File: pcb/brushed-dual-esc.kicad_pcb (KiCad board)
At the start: 2 copper layers, 30 x 25 mm, 33 parts, among them J2 TC2030-NL, J3 DRV1_OUT1, J4 Conn_01x04_Pin, J5 DRV1_OUT2, J6 DRV2_OUT1, J7 DRV2_OUT2, J8 +BATT, J9 -BATT, U1 AZ1117CH-5.0TRG1, U2 TLV77133PDBVR, U3 STM32C011F6U6, U6 DRV8231ADDAR, U7 DRV8231ADDAR

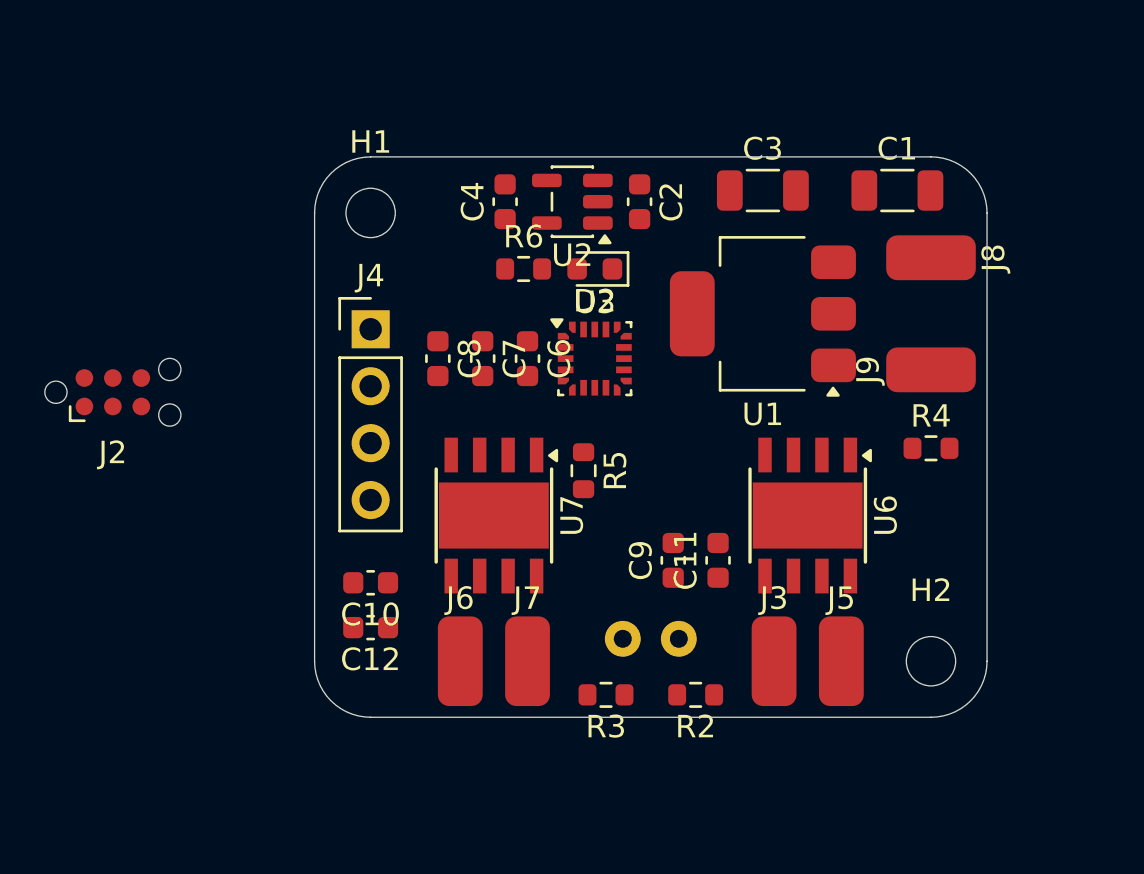
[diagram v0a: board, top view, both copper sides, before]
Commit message: New layout
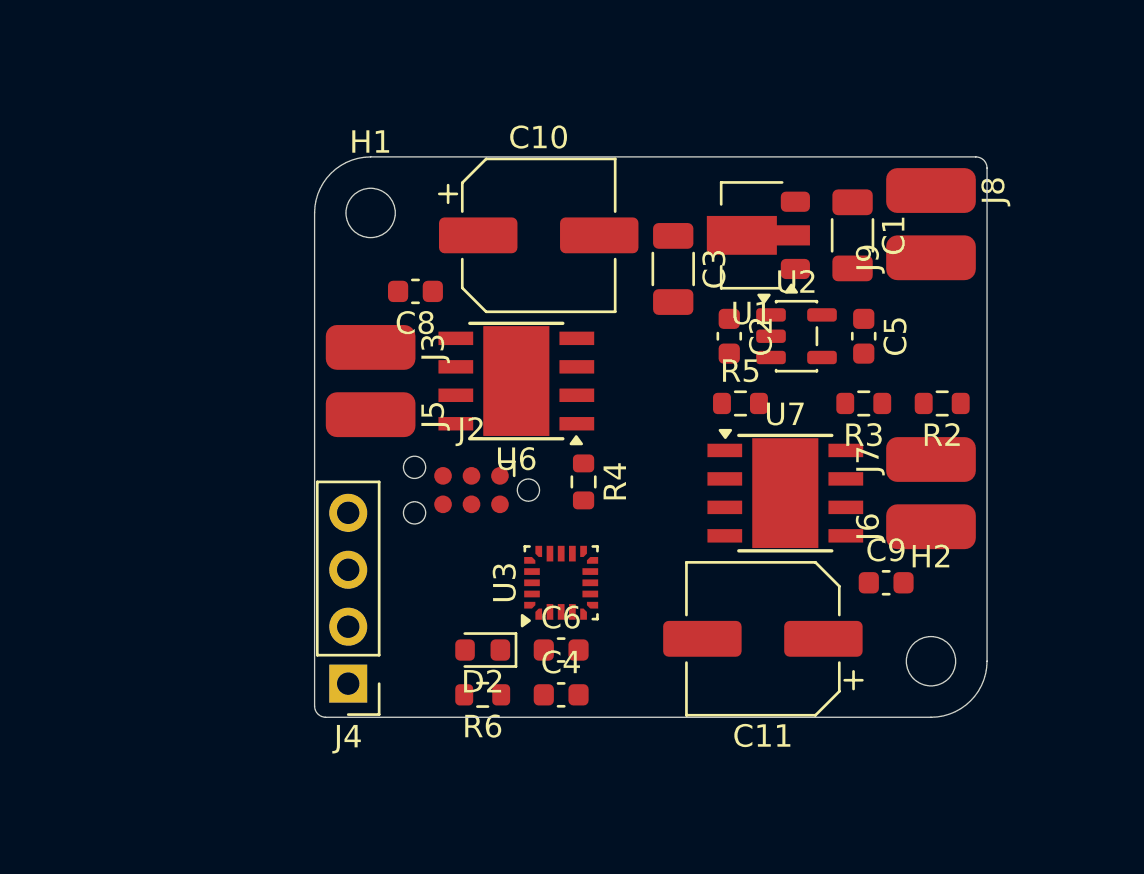
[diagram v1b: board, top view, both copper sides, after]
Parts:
- removed C12, C7: UMK107BJ105KA-T, Capacitor_SMD:C_0603_1608Metric
- C1, C3: value CL21A226KOQNNNG -> CL31A226KAHNNNE
- C10, C11: value UMK107BJ105KA-T -> A768EB107M1ELAS036; footprint Capacitor_SMD:C_0603_1608Metric -> Capacitor_SMD:CP_Elec_6.3x5.7
- C2, C4: value UMK107BJ105KA-T -> 4.7u
- C5: value A750EM337M1CAAE015 -> 4.7u; footprint Capacitor_THT:C_Radial_D6.3mm_H11.0mm_P2.50mm -> Capacitor_SMD:C_0603_1608Metric; moved to F.Cu
- C6, C8, C9: value UMK107BJ105KA-T -> 100n
- U1: value AZ1117CH-5.0TRG1 -> AZ1117CR-5.0TRG1; footprint Package_TO_SOT_SMD:SOT-223-3_TabPin2 -> Package_TO_SOT_SMD:SOT-89-3
- moved J5 23.7 mm to (147.5, 61.5), turned to -90 degrees
- moved J3 22.8 mm to (147.5, 58.5), turned to -90 degrees
- moved C4 22.1 mm to (156.0, 74.0), turned to 0 degrees
- moved J6 21.8 mm to (172.5, 66.5), turned to 90 degrees
- moved J7 20.1 mm to (172.5, 63.5), turned to 90 degrees
- moved R6 19.1 mm to (152.5, 74.0), turned to 180 degrees
- moved D2 17.7 mm to (152.5, 72.0)
- moved R3 17.4 mm to (169.5, 61.0)
- moved C10 17.2 mm to (155.0, 53.5), turned to 0 degrees
- moved R2 17.0 mm to (173.0, 61.0)
- moved J2 16.6 mm to (152.0, 64.9), turned to 180 degrees
- moved J4 15.8 mm to (146.5, 73.5), turned to 180 degrees
- moved C5 15.8 mm to (169.5, 58.0), turned to -90 degrees
- moved R4 15.6 mm to (157.0, 64.5), turned to -90 degrees
- moved U6 14.3 mm to (154.0, 60.0), turned to 180 degrees
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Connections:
- C5 pad 1: +BATT -> +3V3
- C8 pad 1: +3V3 -> +BATT
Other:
- outline, holes or cut-outs redrawn

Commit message: Begin routing
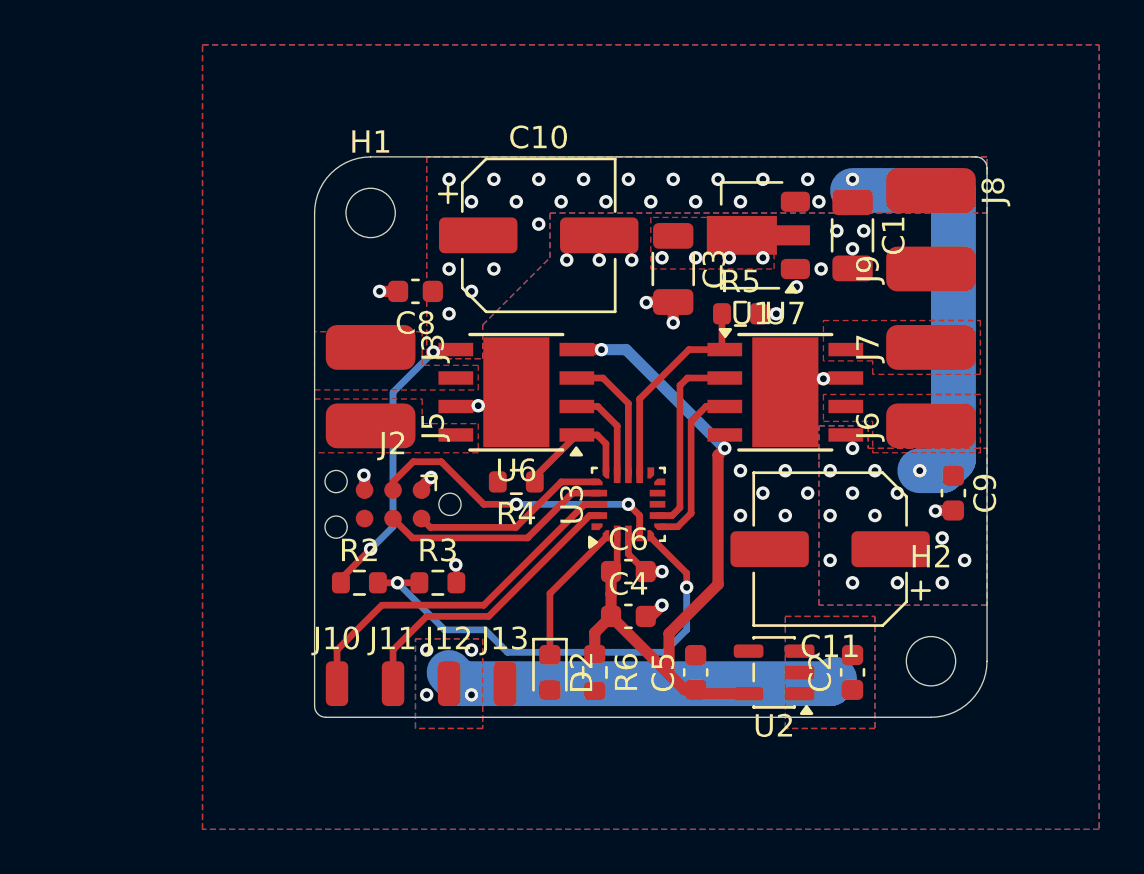
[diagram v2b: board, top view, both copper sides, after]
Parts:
- removed J4: Conn_01x04_Pin, Connector_PinHeader_2.54mm:PinHeader_1x04_P2.54mm_Vertical
- added J10: RX_CH2, Connector_Wire:SolderWirePad_1x01_SMD_1x2mm, F.Cu at (146.0, 73.5)
- added J11: RX_CH1, Connector_Wire:SolderWirePad_1x01_SMD_1x2mm, F.Cu at (148.5, 73.5)
- added J12: +5V, Connector_Wire:SolderWirePad_1x01_SMD_1x2mm, F.Cu at (151.0, 73.5)
- added J13: GND, Connector_Wire:SolderWirePad_1x01_SMD_1x2mm, F.Cu at (153.5, 73.5)
- moved R2 27.2 mm to (147.0, 69.0), turned to 0 degrees
- moved R3 20.6 mm to (150.5, 69.0), turned to 0 degrees
- moved C5 16.8 mm to (162.0, 73.0), turned to 90 degrees
- moved C2 16.0 mm to (169.0, 73.0), turned to 90 degrees
- moved U2 15.0 mm to (165.5, 73.0), turned to 180 degrees
- moved R6 5.10 mm to (157.5, 73.0), turned to -90 degrees
- moved C11 5.00 mm to (168.0, 67.5)
- moved C9 5.00 mm to (173.5, 65.0), turned to -90 degrees
- moved J7 5.00 mm to (172.5, 58.5)
- moved C4 4.61 mm to (159.0, 70.5)
- moved C6 4.61 mm to (159.0, 68.5)
- moved U3 4.61 mm to (159.0, 65.5)
- moved J6 4.50 mm to (172.5, 62.0)
- moved U7 4.50 mm to (166.0, 60.5)
- moved R5 4.00 mm to (164.0, 57.0)
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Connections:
- U3 pad 13: /DRV2_IN2 -> /DRV1_IN1
- U3 pad 14: /DRV2_IN1 -> /DRV1_IN2
- U3 pad 15: /BATT_SENSE -> /DRV1_ISENSE
- U3 pad 5: /DRV1_ISENSE -> /BATT_SENSE
- U3 pad 6: /DRV1_IN1 -> /DRV2_IN1
- U3 pad 7: /DRV1_IN2 -> /DRV2_IN2
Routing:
- net +3V3: track 0.00 -> 33.6 mm, vias 0 -> 3
- net +BATT: track 0.00 -> 31.3 mm, vias 0 -> 39
- net /BATT_SENSE: track 0.00 -> 21.2 mm, vias 0 -> 2
- net +5V: track 0.00 -> 17.5 mm, vias 0 -> 8
- net /RX_CH2: track 0.00 -> 15.9 mm
- net GND: track 0.00 -> 15.6 mm, vias 0 -> 25
- net /~{RESET}: track 0.00 -> 13.5 mm, vias 0 -> 2
- net /RX_CH1: track 0.00 -> 13.2 mm
- net /SWCLK: track 0.00 -> 10.4 mm
- net /DRV2_ISENSE: track 0.00 -> 9.76 mm
- net /SWDIO: track 0.00 -> 8.77 mm
- net /DRV2_IN2: track 0.00 -> 8.73 mm
- net /DRV2_IN1: track 0.00 -> 7.45 mm
- net /LED: track 0.00 -> 6.27 mm
- net /DRV1_IN1: track 0.00 -> 5.97 mm
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- added copper zone on B.Cu, net +5V
- added copper zone on F.Cu, net +5V
- added copper zone on B.Cu, net +BATT
- added copper zone on F.Cu, net +BATT
- added copper zone on F.Cu, net /DRV1_OUT1
- added copper zone on F.Cu, net /DRV1_OUT2
- added copper zone on F.Cu, net /DRV2_OUT1
- added copper zone on F.Cu, net /DRV2_OUT2
- added copper zone on B.Cu, net GND
- added copper zone on F.Cu, net GND

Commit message: Finish this diabolical routing
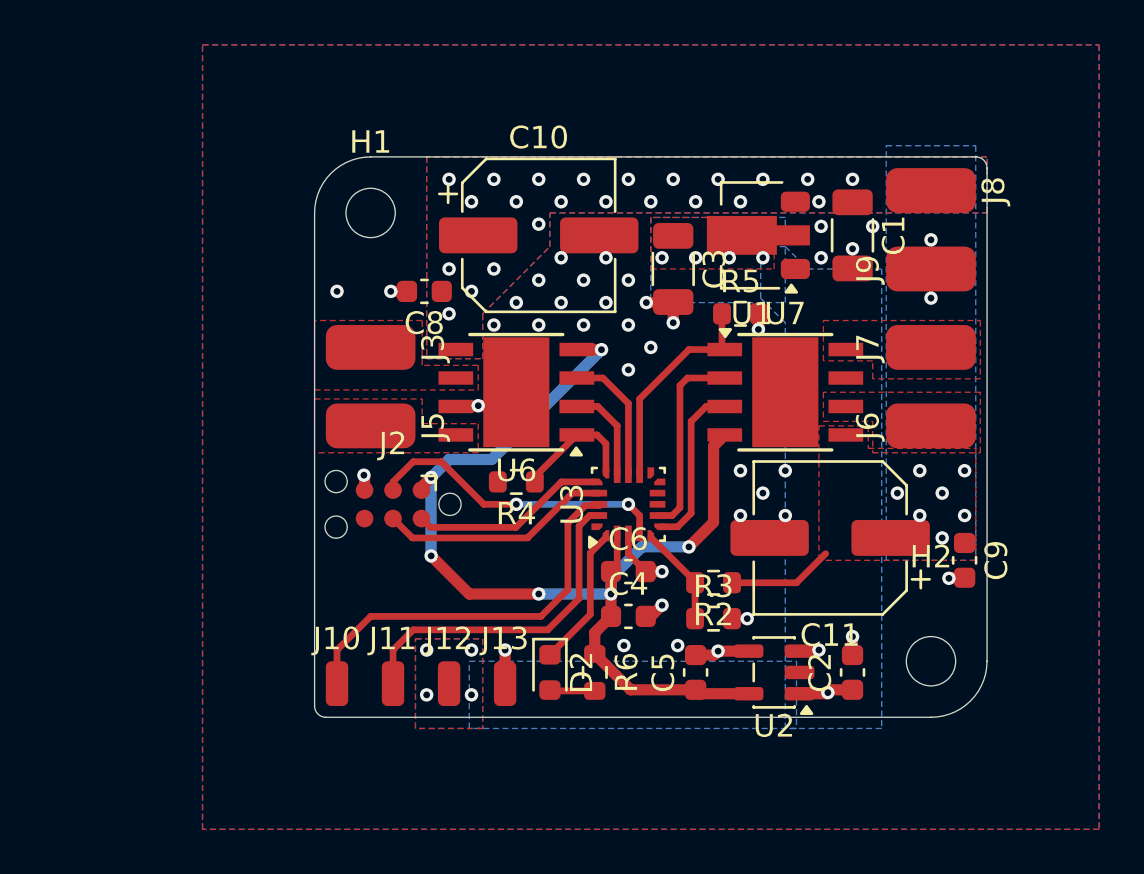
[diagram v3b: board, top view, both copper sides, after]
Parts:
- moved R2 15.8 mm to (162.8, 69.0), turned to 180 degrees
- moved R3 12.4 mm to (162.8, 70.6)
- moved C9 3.04 mm to (174.0, 68.0)
- moved C11 0.50 mm to (168.0, 67.0)
- moved C8 0.40 mm to (149.9, 56.0)
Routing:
- net +BATT: track 31.3 -> 4.71 mm, vias 39 -> 30
- net /BATT_SENSE: track 21.2 -> 4.44 mm, vias 2 -> 0
- net +3V3: track 33.6 -> 47.9 mm, vias 3 -> 6
- net +5V: track 17.5 -> 3.32 mm, vias 8 -> 10
- net Net-(D2-A): track 0.00 -> 2.02 mm
- net /RX_CH1: track 13.2 -> 15.1 mm
- net /RX_CH2: track 15.9 -> 17.7 mm
- net GND: track 15.6 -> 17.0 mm, vias 25 -> 41
